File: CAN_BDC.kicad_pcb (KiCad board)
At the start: 2 copper layers, 24 x 28.5 mm, 35 parts, among them P1 CONN_01X02, P2 CONN_01X05, P3 CONN_01X02, P4 CONN_01X02, P5 CONN_01X02, P6 CONN_01X02, P7 CONN_01X04, P8 CONN_01X01, P9 CONN_01X02, U1 PSD2CAN, U2 SN65HVD232D, U3 POLOLU_A4988, U4 STM32F042G4U6, U5 MC33063

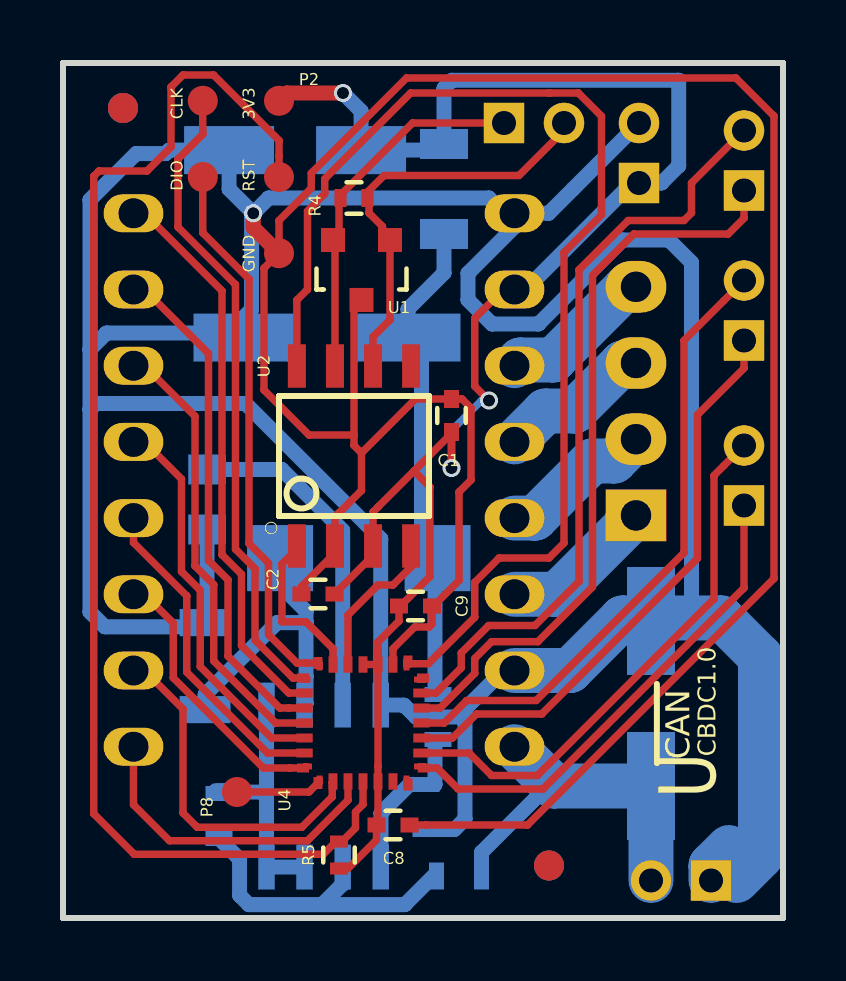
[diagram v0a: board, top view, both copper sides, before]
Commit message: Buck-converter update.
Buck-converter update.
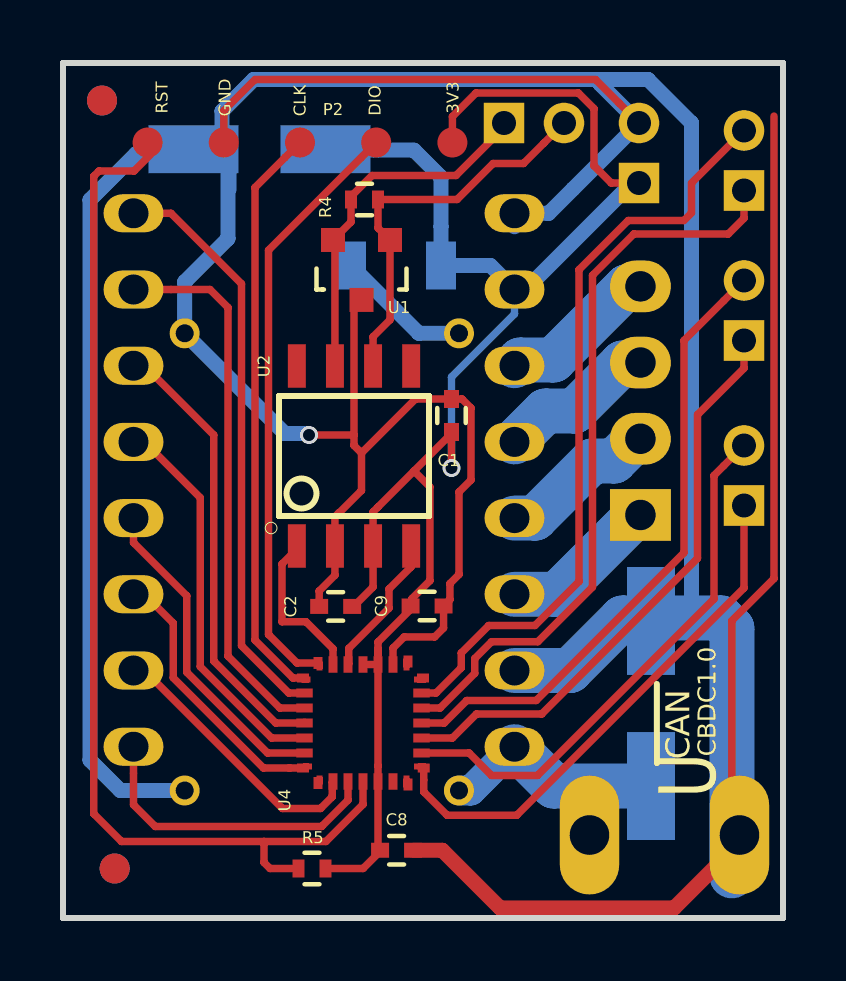
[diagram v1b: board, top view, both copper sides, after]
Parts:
- removed C5: 470p, Capacitors_SMD:C_0805
- removed C6: 330u, Capacitors_SMD:c_elec_6.3x7.7
- removed D1: 1N5819, Resistors_SMD:R_1206
- removed L1: 220uH, usb_ccb_custom:DE0704_Coil_2
- removed P8: CONN_01X01, usb_ccb_custom:smd1Conn
- removed R1: 2,2k, Resistors_SMD:R_0603
- removed R2: 0.33, Resistors_SMD:R_0603
- removed R3: 3,9k, Resistors_SMD:R_0603
- removed R6: 0, Resistors_SMD:R_0603
- P2: footprint usb_ccb_custom:swd_smd_conn5_x2 -> usb_ccb_custom:swd_smd_conn5
- P6: footprint Pin_Headers:Pin_Header_Straight_1x02_Pitch2.00mm -> usb_ccb_custom:AK300-2MIRROR
- U5: value MC33063 -> Mini-360; footprint usb_ccb_custom:SOIC-8 -> usb_ccb_custom:Mini-360
- moved f1 14.5 mm to (140.2, 109.9)
- moved f3 14.5 mm to (140.2, 109.9)
- moved U5 4.52 mm to (151.7, 107.3), turned to 90 degrees
- moved L2 3.01 mm to (149.6, 89.8), turned to 0 degrees
- moved P2 2.41 mm to (147.7, 85.7), turned to 180 degrees
- moved P6 1.79 mm to (161.1, 108.8), turned to 180 degrees
- moved C7 1.19 mm to (145.0, 85.9)
- moved R5 1.01 mm to (146.8, 109.9), turned to 0 degrees
- moved C8 0.85 mm to (149.6, 109.3)
- moved f2 0.74 mm to (139.8, 84.3)
- moved f4 0.74 mm to (139.8, 84.3)
- moved C2 0.72 mm to (147.6, 101.2)
- moved C9 0.39 mm to (150.6, 101.2)
- moved R4 0.35 mm to (148.6, 87.6)
- moved P7 0.15 mm to (157.7, 98.1)
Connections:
- L2 pad 1: Net-(C6-Pad1) -> Net-(L2-Pad1)
- P2 pad 2: Net-(P2-Pad2) -> SW_DIO
- P2 pad 3: GND -> SW_CLK
- P2 pad 4: SW_CLK -> GND
- P2 pad 5: SW_DIO -> Net-(P2-Pad5)
- P6 pad 1: GND -> VPP
- P6 pad 2: VPP -> GND
- R5 pad 1: Net-(P2-Pad2) -> Net-(P2-Pad5)
- U2 pad 5: Net-(U2-Pad5) -> (no net)
- U4 pad 4: Net-(P2-Pad2) -> Net-(P2-Pad5)
- U4 pad 6: Net-(U4-Pad6) -> (no net)
- U5 pad 1: Net-(R2-Pad1) -> VPP
- U5 pad 2: Net-(D1-Pad1) -> GND
- U5 pad 3: Net-(C5-Pad1) -> Net-(L2-Pad1)
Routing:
- net Net-(P2-Pad2): track 43.4 -> 0.00 mm
- net CAN_MOD: track 40.1 -> 0.42 mm
- net Net-(P2-Pad5): track 0.00 -> 36.0 mm
- net GND: track 212.1 -> 183.4 mm
- net Net-(C6-Pad1): track 16.7 -> 0.00 mm
- net Net-(C5-Pad1): track 11.2 -> 0.00 mm
- net Net-(R2-Pad2): track 10.7 -> 0.00 mm
- net Net-(D1-Pad1): track 9.43 -> 0.00 mm
- net Net-(R2-Pad1): track 8.94 -> 0.00 mm
- net Net-(R1-Pad1): track 5.54 -> 0.00 mm
- net Net-(L2-Pad1): track 0.00 -> 4.54 mm
- net Net-(U4-Pad1): track 2.82 -> 0.00 mm
- net DRV_MS1: track 11.9 -> 9.35 mm
- net SW_CLK: track 21.5 -> 19.3 mm
- net VPP: track 12.1 -> 10.1 mm
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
